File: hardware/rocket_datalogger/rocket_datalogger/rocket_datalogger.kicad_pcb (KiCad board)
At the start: 2 copper layers, 70 x 55 mm, 79 parts, among them J1 AMP_Superseal_9-6437287-8, J2 TC2030, U1 STM32F042K6Ux, U2 TLE42744DV33ATMA1, U3 TCAN3403DRQ1, U4 R-78E5.0-0.5, Y1 ECS-160-10-36Q-AES-TR

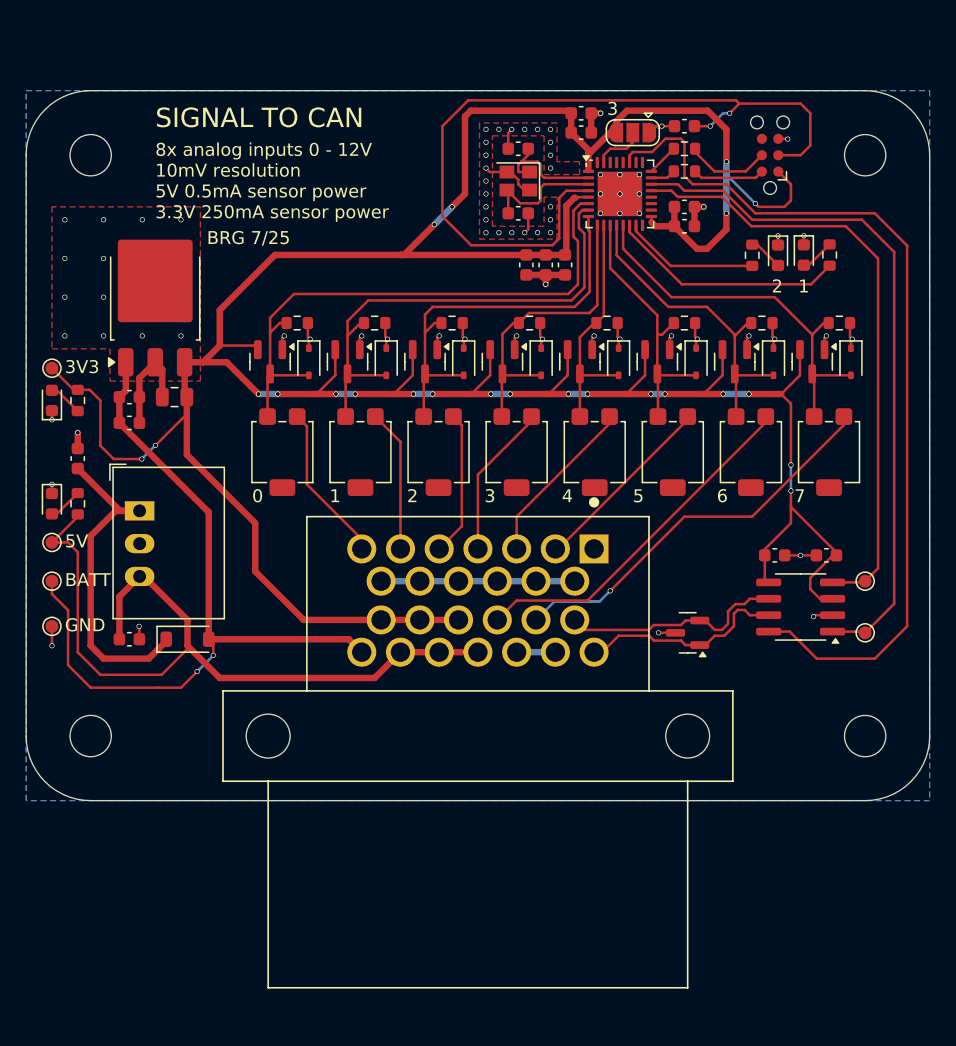
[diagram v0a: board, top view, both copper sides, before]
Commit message: PCB design rev 1
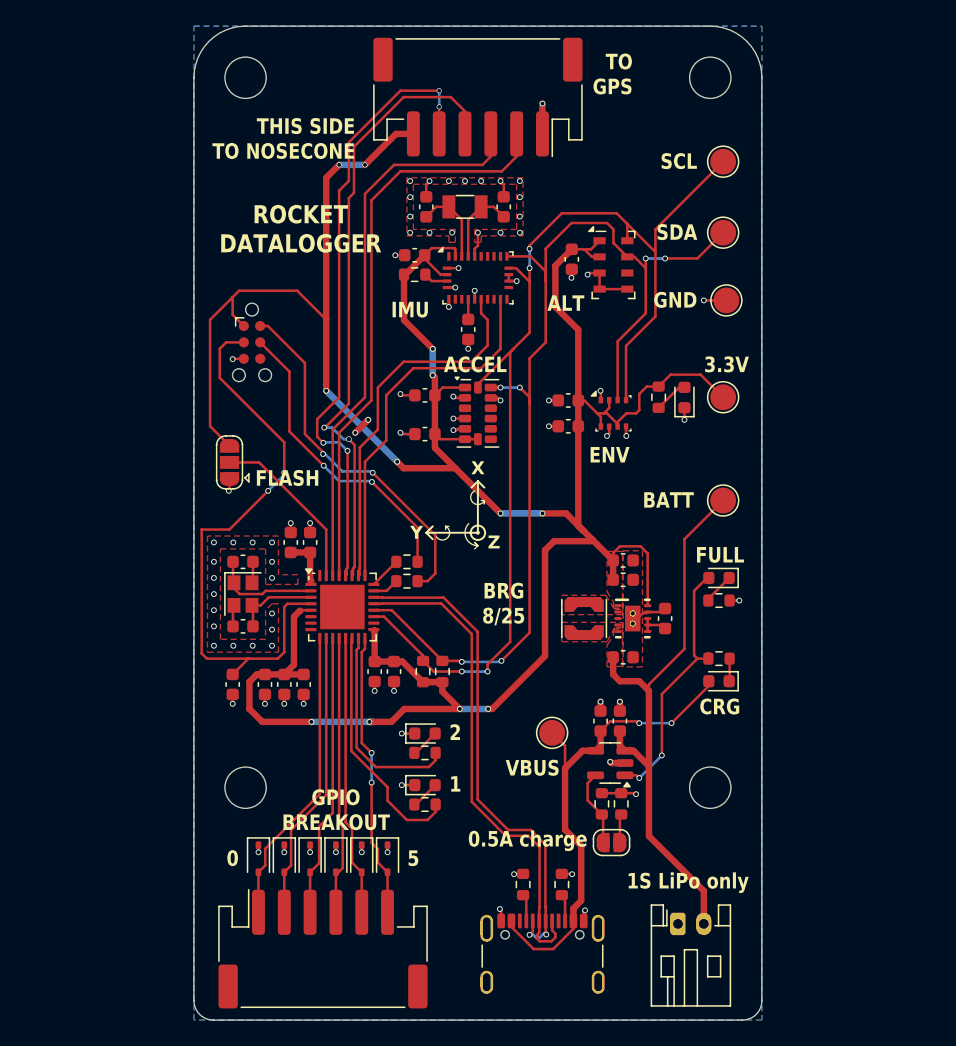
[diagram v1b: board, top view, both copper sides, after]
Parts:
- removed D12, D17, D18, D19, D20: BAT54S, Package_TO_SOT_SMD:SOT-23
- removed D13, D14, D15, D16: PESD3V3L1BA, Diode_SMD:D_SOD-323
- removed D21: CDBW140-G, Diode_SMD:D_SOD-123
- removed D22: LED, LED_SMD:LED_0603_1608Metric
- removed J1: AMP_Superseal_9-6437287-8, signal_to_can:TE_9-6437287-8_1
- removed RV1, RV2, RV3, RV4, RV5, RV6, RV7, RV8: 3314G-1-503E, Potentiometer_SMD:Potentiometer_Bourns_3314G_Vertical
- added C18: 0.1uF, Capacitor_SMD:C_0603_1608Metric, F.Cu at (157.0, 99.0)
- added C19: 0.1uF, Capacitor_SMD:C_0603_1608Metric, F.Cu at (157.0, 101.0)
- added C20: 1uF Tantalum, Capacitor_SMD:C_0603_1608Metric, F.Cu at (145.9, 101.6)
- added C21: 0.1uF, Capacitor_SMD:C_0603_1608Metric, F.Cu at (145.1, 87.8)
- added C22: 0.1uF, Capacitor_SMD:C_0603_1608Metric, F.Cu at (145.9, 98.6)
- added C23: 0.1uF, Capacitor_SMD:C_0603_1608Metric, F.Cu at (149.2, 93.5)
- added C24: 22 pF, Capacitor_SMD:C_0603_1608Metric, F.Cu at (152.0, 84.0)
- added C25: 22 pF, Capacitor_SMD:C_0603_1608Metric, F.Cu at (146.0, 84.0)
- added J3: TC2030, Connector:Tag-Connect_TC2030-IDC-NL_2x03_P1.27mm_Vertical, F.Cu at (132.5, 94.5)
- added J4: JST-PH 1x2, Connector_JST:JST_PH_S2B-PH-K_1x02_P2.00mm_Horizontal, F.Cu at (165.5, 139.6)
- added J5: USB_C_Receptacle_USB2.0_16P, Connector_USB:USB_C_Receptacle_GCT_USB4105-xx-A_16P_TopMnt_Horizontal, F.Cu at (155.0, 143.0)
- added J6: JST-PH-S6B-SM4_TB, Connector_JST:JST_PH_S6B-PH-SM4-TB_1x06-1MP_P2.00mm_Horizontal, F.Cu at (150.0, 75.5)
- added JP2: Jumper_2_Open, Jumper:SolderJumper-2_P1.3mm_Open_RoundedPad1.0x1.5mm, F.Cu at (160.3, 133.2)
- added L1: 1.5uH LPS3015-152MRC, Inductor_SMD:L_Coilcraft_LPS3010, F.Cu at (158.2, 115.9)
- added U5: BME280, Package_LGA:Bosch_LGA-8_2.5x2.5mm_P0.65mm_ClockwisePinNumbering, F.Cu at (160.5, 100.0)
- added U7: ~, Package_LGA:LGA-14_3x5mm_P0.8mm_LayoutBorder1x6y, F.Cu at (150.0, 100.0)
- added U8: BNO055, Package_LGA:LGA-28_5.2x3.8mm_P0.5mm, F.Cu at (150.0, 89.5)
- added Y2: ECX-.327-CDX-1293, Crystal:Crystal_SMD_3215-2Pin_3.2x1.5mm, F.Cu at (149.0, 84.0)
- C1: value 4.7uF -> 0.1uF
- C11: value 1uF -> 10 uF
- C13: value 22uF -> 10uF; footprint Capacitor_SMD:C_0805_2012Metric -> Capacitor_SMD:C_0603_1608Metric
- C14: value 0.1uF -> 10uF
- C15: value 0.1uF -> 10uF 6.3V
- C16: value 10uF -> 10uF 6.3V
- C17: value 10uF -> 0.1uF
- C3: value 0.1uF -> 4.7uF
- D1, D2, D3: value LED -> PESD3V3L1BA; footprint LED_SMD:LED_0603_1608Metric -> Diode_SMD:D_SOD-323
- D10: value BAT54S -> Red LED; footprint Package_TO_SOT_SMD:SOT-23 -> LED_SMD:LED_0603_1608Metric
- D11: value BAT54S -> Green LED; footprint Package_TO_SOT_SMD:SOT-23 -> LED_SMD:LED_0603_1608Metric
- D4: value NUP2105L -> PESD3V3L1BA; footprint Package_TO_SOT_SMD:SOT-23 -> Diode_SMD:D_SOD-323
- D7, D8: value PESD3V3L1BA -> LED; footprint Diode_SMD:D_SOD-323 -> LED_SMD:LED_0603_1608Metric
- D9: value BAT54S -> LED; footprint Package_TO_SOT_SMD:SOT-23 -> LED_SMD:LED_0603_1608Metric
- J2: value TC2030 -> JST-PH-S6B-SM4_TB; footprint Connector:Tag-Connect_TC2030-IDC-NL_2x03_P1.27mm_Vertical -> Connector_JST:JST_PH_S6B-PH-SM4-TB_1x06-1MP_P2.00mm_Horizontal
- R1, R2: value 22 -> 5.1k
- R10: value 6.8k -> 2.2k
- R11: value 6.8k -> 10k
- R12, R13: value 6.8k -> 470
- R14: value 1k -> 10k
- R5: value 1k -> 22
- R6: value 6.8k -> 22
- R7, R8: value 6.8k -> 4.7k
- R9: value 6.8k -> 1k
- TP1: value POWER_INPUT -> TestPoint; footprint TestPoint:TestPoint_Pad_D1.0mm -> TestPoint:TestPoint_Pad_D2.0mm
- TP2: value GND -> BATT; footprint TestPoint:TestPoint_Pad_D1.0mm -> TestPoint:TestPoint_Pad_D2.0mm
- TP3: value 3.3V -> 3V3; footprint TestPoint:TestPoint_Pad_D1.0mm -> TestPoint:TestPoint_Pad_D2.0mm
- TP4: value CAN_TX -> GND; footprint TestPoint:TestPoint_Pad_D1.0mm -> TestPoint:TestPoint_Pad_D2.0mm
- TP5: value CAN_RX -> SCL; footprint TestPoint:TestPoint_Pad_D1.0mm -> TestPoint:TestPoint_Pad_D2.0mm
- TP6: value TestPoint -> SDA; footprint TestPoint:TestPoint_Pad_D1.0mm -> TestPoint:TestPoint_Pad_D2.0mm
- U2: value TLE42744DV33ATMA1 -> ~; footprint Package_TO_SOT_SMD:TO-252-3_TabPin2 -> rocket_datalogger:DSK0010A
- U3: value TCAN3403DRQ1 -> MCP73831-2-OT; footprint Package_SO:SOIC-8_3.9x4.9mm_P1.27mm -> Package_TO_SOT_SMD:SOT-23-5
- U4: value R-78E5.0-0.5 -> MS5607-02BA; footprint Converter_DCDC:Converter_DCDC_RECOM_R-78E-0.5_THT -> Package_LGA:LGA-8_3x5mm_P1.25mm
- moved J2 70.6 mm to (138.0, 141.5), turned to 0 degrees
- moved H2 70.0 mm to (168.0, 74.0)
- moved H3 68.6 mm to (132.0, 129.0)
- moved D1 63.0 mm to (133.0, 134.5)
- moved D2 60.4 mm to (135.0, 134.5)
- moved R2 58.4 mm to (153.5, 136.5), turned to 90 degrees
- moved TP6 57.3 mm to (169.0, 86.0)
- moved R1 56.1 mm to (156.5, 136.5), turned to 90 degrees
- moved TP2 52.9 mm to (169.0, 106.8)
- moved R3 52.9 mm to (145.9, 130.3), turned to 180 degrees
- moved TP3 52.0 mm to (169.0, 98.8)
- moved C1 50.9 mm to (131.0, 121.0), turned to -90 degrees
- moved C16 46.7 mm to (161.0, 123.8)
- moved R4 46.1 mm to (145.9, 126.3), turned to 180 degrees
- moved C2 45.6 mm to (143.5, 120.0), turned to -90 degrees
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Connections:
- C1 pad 1: +3V3 -> /Microcontroller/NRST
- C10 pad 1: +3V3 -> +3.3V
- C11 pad 1: GND -> +BATT
- C11 pad 2: +BATT -> GND
- C12 pad 1: GND -> Net-(U2-EN)
- C12 pad 2: +BATT -> GND
- C13 pad 1: +3V3 -> +3.3V
- C14 pad 1: +3V3 -> +3.3V
- C15 pad 1: +3V3 -> VBUS
- C16 pad 1: Net-(D21-K) -> +BATT
- C17 pad 1: +5V -> +3.3V
- C2 pad 1: +3V3 -> +3.3V
- C3 pad 1: /Microcontroller/NRST -> +3.3V
- C4 pad 1: +3V3 -> +3.3V
- C5 pad 1: +3V3 -> +3.3V
- C6 pad 1: +3V3 -> +3.3V
- C8 pad 1: +3V3 -> +3.3V
- D1 pad 2: Net-(D1-A) -> /GPIO_0
- D10 pad 1: GND -> Net-(D10-K)
- D10 pad 2: +3V3 -> VBUS
- D11 pad 1: GND -> Net-(D11-K)
- D11 pad 2: +3V3 -> /USB-C LiPo Charging/STAT
- D2 pad 2: Net-(D2-A) -> /GPIO_1
- D3 pad 2: Net-(D3-A) -> /GPIO_2
- D4 pad 1: /CAN_P -> GND
- D4 pad 2: /CAN_N -> /GPIO_3
- D5 pad 2: /3.3V_ANALOG_INPUT_0 -> /GPIO_4
- D6 pad 2: /3.3V_ANALOG_INPUT_1 -> /GPIO_5
- D7 pad 2: /3.3V_ANALOG_INPUT_2 -> Net-(D7-A)
- D8 pad 2: /3.3V_ANALOG_INPUT_3 -> Net-(D8-A)
- D9 pad 2: +3V3 -> Net-(D9-A)
- J2 pad 1: +3V3 -> /GPIO_0
- J2 pad 2: Net-(J2-Pin_2) -> /GPIO_1
- J2 pad 3: /Microcontroller/NRST -> /GPIO_2
- J2 pad 4: Net-(J2-Pin_4) -> /GPIO_3
- J2 pad 5: GND -> /GPIO_4
- J2 pad 6: unconnected-(J2-Pin_6-Pad6) -> /GPIO_5
- JP1 pad 3: +3V3 -> +3.3V
- R1 pad 1: Net-(J2-Pin_2) -> Net-(J5-CC2)
- R1 pad 2: /Microcontroller/SWDIO -> GND
- R10 pad 1: /3.3V_ANALOG_INPUT_4 -> Net-(JP2-A)
- R11 pad 1: /3.3V_ANALOG_INPUT_5 -> Net-(JP2-B)
- R12 pad 1: /3.3V_ANALOG_INPUT_6 -> Net-(D10-K)
- R12 pad 2: GND -> /USB-C LiPo Charging/STAT
- R13 pad 1: /3.3V_ANALOG_INPUT_7 -> Net-(D11-K)
- R14 pad 1: +5V -> +3.3V
- R2 pad 1: Net-(J2-Pin_4) -> Net-(J5-CC1)
- R2 pad 2: /Microcontroller/SWCLK -> GND
- R3 pad 2: Net-(D1-A) -> Net-(D7-A)
- R4 pad 2: Net-(D2-A) -> Net-(D8-A)
- R5 pad 1: +3V3 -> Net-(J3-Pin_2)
- R5 pad 2: Net-(D3-A) -> /Microcontroller/SWDIO
- R6 pad 1: /3.3V_ANALOG_INPUT_0 -> Net-(J3-Pin_4)
- R6 pad 2: GND -> /Microcontroller/SWCLK
- R7 pad 1: /3.3V_ANALOG_INPUT_1 -> +3.3V
- R7 pad 2: GND -> /SDA
- R8 pad 1: /3.3V_ANALOG_INPUT_2 -> +3.3V
- R8 pad 2: GND -> /SCL
- R9 pad 1: /3.3V_ANALOG_INPUT_3 -> +3.3V
- R9 pad 2: GND -> Net-(D9-A)
- TP1 pad 1: +BATT -> VBUS
- TP2 pad 1: GND -> +BATT
- TP3 pad 1: +3V3 -> +3.3V
- TP4 pad 1: /CAN_TX -> GND
- TP5 pad 1: /CAN_RX -> /SCL
- TP6 pad 1: +5V -> /SDA
- U1 pad 1: +3V3 -> +3.3V
- U1 pad 10: /3.3V_ANALOG_INPUT_4 -> /GPIO_1
- U1 pad 11: /3.3V_ANALOG_INPUT_5 -> /GPIO_2
- U1 pad 12: /3.3V_ANALOG_INPUT_6 -> /GPIO_3
- U1 pad 13: /3.3V_ANALOG_INPUT_7 -> /GPIO_4
- U1 pad 16: unconnected-(U1-PB2-Pad16) -> /GPIO_5
- U1 pad 17: +3V3 -> +3.3V
- U1 pad 19: unconnected-(U1-PA9-Pad19) -> /SCL
- U1 pad 20: unconnected-(U1-PA10-Pad20) -> /SDA
- U1 pad 21: /CAN_RX -> /USB_D_N
- U1 pad 22: /CAN_TX -> /USB_D_P
- U1 pad 25: unconnected-(U1-PA15-Pad25) -> /IMU_INT
- U1 pad 26: unconnected-(U1-PB3-Pad26) -> /~IMU_RESET
- U1 pad 27: /CAN_STANDBY -> /GPS_TIMEPULSE
- U1 pad 28: unconnected-(U1-PB5-Pad28) -> /GPS_RESET
- U1 pad 29: unconnected-(U1-PB6-Pad29) -> /UART_TX
- U1 pad 30: unconnected-(U1-PB7-Pad30) -> /UART_RX
- U1 pad 5: +3V3 -> +3.3V
- U1 pad 6: /3.3V_ANALOG_INPUT_0 -> unconnected-(U1-PA0-Pad6)
- U1 pad 7: /3.3V_ANALOG_INPUT_1 -> unconnected-(U1-PA1-Pad7)
- U1 pad 8: /3.3V_ANALOG_INPUT_2 -> unconnected-(U1-PA2-Pad8)
- U1 pad 9: /3.3V_ANALOG_INPUT_3 -> /GPIO_0
- U2 pad 1: +BATT -> +3.3V
- U2 pad 2: GND -> Net-(U2-L2)
- U2 pad 3: +3V3 -> GND
- U3 pad 1: /CAN_TX -> /USB-C LiPo Charging/STAT
- U3 pad 3: +3V3 -> +BATT
- U3 pad 4: /CAN_RX -> VBUS
- U3 pad 5: +3V3 -> Net-(JP2-B)
- U4 pad 1: Net-(D21-K) -> +3.3V
- U4 pad 2: GND -> +3.3V
- U4 pad 3: +5V -> GND
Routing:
- net +3V3: track 263.7 -> 0.00 mm, vias 23 -> 0
- net +3.3V: track 0.00 -> 226.5 mm, vias 0 -> 12
- net /SCL: track 0.00 -> 86.4 mm, vias 0 -> 4
- net /SDA: track 0.00 -> 82.3 mm, vias 0 -> 6
- net /CAN_STANDBY: track 69.7 -> 0.00 mm
- net +5V: track 60.4 -> 0.00 mm
- net /CAN_TX: track 54.0 -> 0.00 mm
- net /GPS_RESET: track 0.00 -> 48.4 mm, vias 0 -> 4
- net /GPS_TIMEPULSE: track 0.00 -> 48.2 mm, vias 0 -> 2
- net /CAN_RX: track 47.7 -> 0.00 mm
- net /3.3V_ANALOG_INPUT_0: track 44.5 -> 0.00 mm
- net /UART_TX: track 0.00 -> 44.5 mm
- net /UART_RX: track 0.00 -> 43.3 mm
- net /USB_D_P: track 0.00 -> 38.6 mm, vias 0 -> 2
- net /USB_D_N: track 0.00 -> 38.5 mm
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- added copper zone on F.Cu, net +3.3V
- added copper zone on F.Cu, net +BATT
- added copper zone on F.Cu, net Net-(U2-L1)
- added copper zone on F.Cu, net Net-(U2-L2)
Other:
- board size 70 x 55 mm -> 44 x 77 mm
- board text added: "0.5A charge"
- board text added: "1S LiPo only"
- board text added: "3.3V"
- board text added: "ACCEL"
- board text added: "ALT"
- board text added: "BRG 8/25"
- board text added: "CRG"
- board text added: "ENV"
- board text added: "FLASH"
- board text added: "FULL"
- board text added: "GPIO BREAKOUT"
- board text added: "IMU"
- board text added: "ROCKET DATALOGGER"
- board text added: "SCL"
- board text added: "SDA"
- board text added: "THIS SIDE TO NOSECONE"
- board text added: "TO GPS"
- board text added: "VBUS"
- board text added: "X"
- board text added: "Y"
- board text added: "Z"
- board text added: "roket go brr"
- board text removed: "3"
- board text removed: "3V3"
- board text removed: "4"
- board text removed: "5V"
- board text removed: "6"
- board text removed: "7"
- board text removed: "8x analog inputs 0 - 12V 10mV resolution 5V 0.5mA sensor power 3.3V 250mA sensor power"
- board text removed: "BRG 7/25"
- board text removed: "SIGNAL TO CAN"
